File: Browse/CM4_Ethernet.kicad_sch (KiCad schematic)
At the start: 6 parts

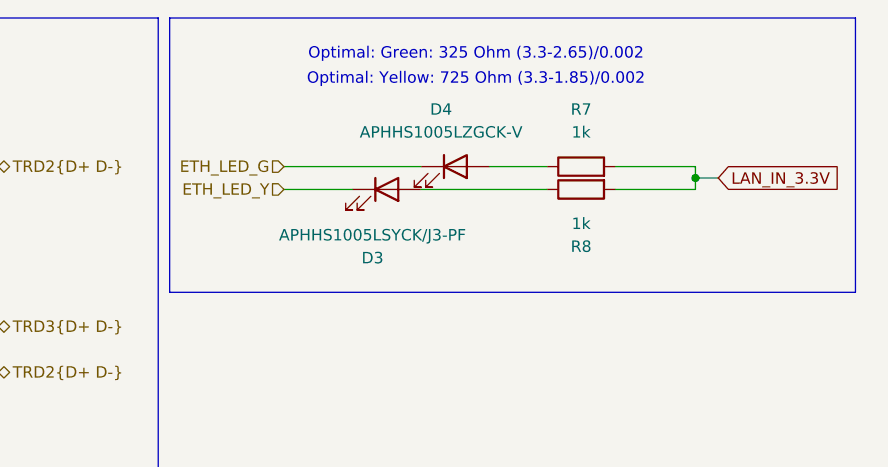
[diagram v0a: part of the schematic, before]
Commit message: Deploying to gh-pages from @ Nautilus-UUV/nautilus-mainboard-PCB@a81f7ffbfc5f9b51f47d7f388c30fcea2673b9ea 🚀
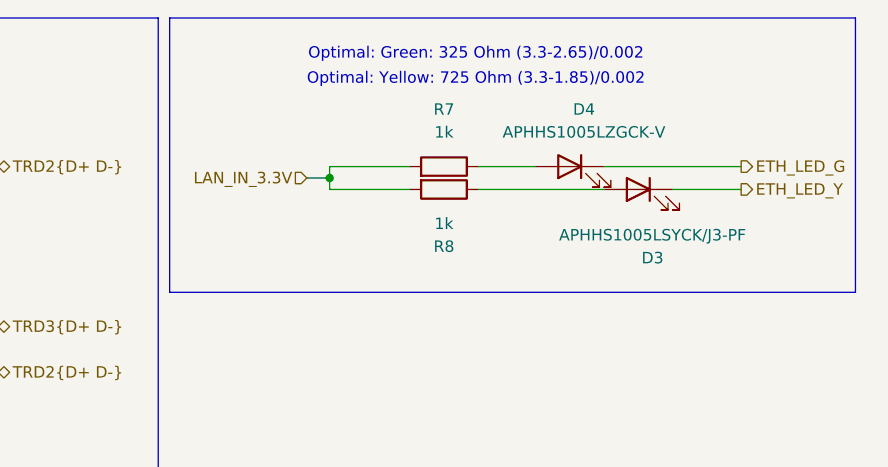
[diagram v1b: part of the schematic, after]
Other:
- moved on the sheet: D3, D4, R7, R8

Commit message: Deploying to gh-pages from @ Nautilus-UUV/nautilus-mainboard-PCB@2d3890115fd9d3c0bb909c9898aa64801bed9e67 🚀
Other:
- company: (none) -> Davide
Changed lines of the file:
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@@
 (kicad_sch (version 20250114) (generator "eeschema") (generator_version "9.0")
   (paper "A4")
+  (title_block
+    (date "2025-11-18")
+    (company "Davide")
+  )
   (junction (at 134.62 54.61) (diameter 0) (color 0 0 0 0)
   )
